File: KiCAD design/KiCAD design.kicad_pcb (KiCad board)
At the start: 2 copper layers, 94 x 84 mm, 31 parts, among them J201 Conn_02x19_Odd_Even, J202 Conn_01x03_Female, J203 Conn_01x03_Female, J204 Conn_02x19_Odd_Even, J205 JST BATTERY, J206 JST SENS TOF 2, J208 JST SENS TOF 1, J401 Conn_02x06_Top_Bottom, U101 NUCLEO64-F411RE, U301 MCP1804T, U302 MIC5317, U401 ACS712xLCTR-20A

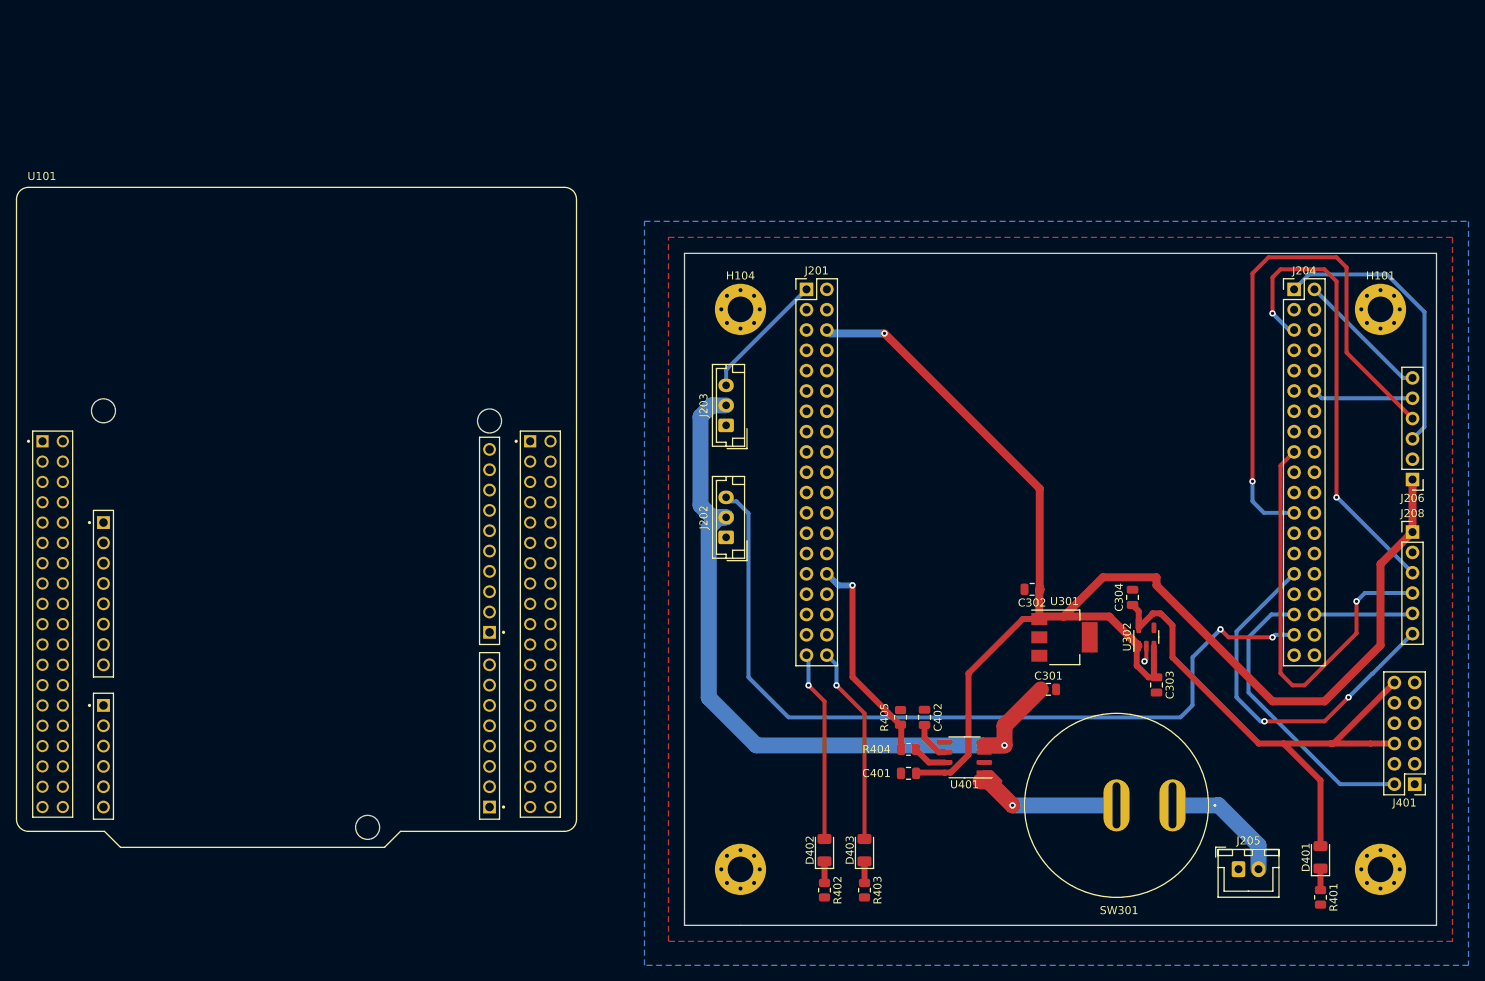
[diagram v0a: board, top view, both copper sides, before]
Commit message: end PCB
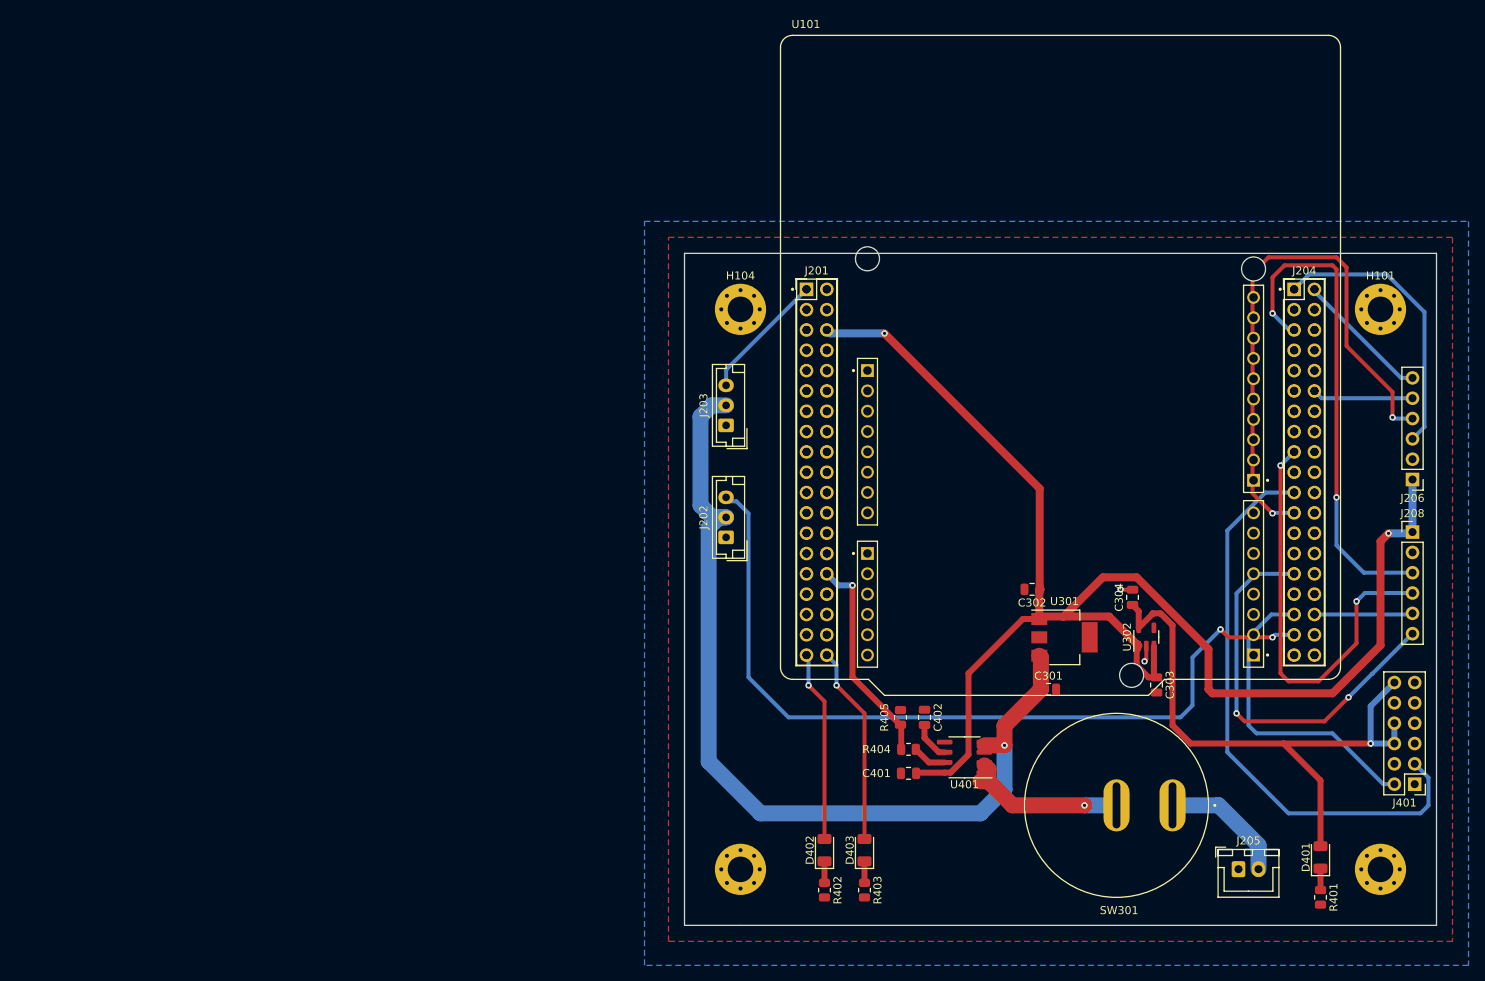
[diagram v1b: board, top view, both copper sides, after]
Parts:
- moved U101 97.4 mm to (150.0, 67.0)
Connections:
- J201 pad 16: unconnected-(J201-Pad16) -> /CONNECTORS/BT_3.3V
- J401 pad 8: /CONNECTORS/RST_N -> +3.3V
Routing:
- net /CONNECTORS/Bluetooth_TX: track 0.00 -> 72.7 mm
- net +12V: track 93.5 -> 112.7 mm
- net /CONNECTORS/TOF1_SDA: track 57.5 -> 62.3 mm
- net +3.3V: track 71.9 -> 76.0 mm, vias 0 -> 1
- net /CONNECTORS/TOF1_DATA_READY: track 46.2 -> 50.2 mm
- net +5V: track 178.5 -> 181.7 mm, vias 1 -> 2
- net /CONNECTORS/Bluetooth_RX: track 36.8 -> 39.2 mm
- net GND: track 2.01 -> 3.53 mm, vias 1 -> 2
- net /CONNECTORS/TOF2_SCL: track 69.7 -> 70.6 mm, vias 1 -> 2
- net /ON_BOARD_COMPONENTS/IP+: track 20.7 -> 21.4 mm
- net /CONNECTORS/TOF1_SCL: track 52.6 -> 52.9 mm, vias 1 -> 2
